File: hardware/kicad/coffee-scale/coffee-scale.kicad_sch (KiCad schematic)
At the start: 0 parts

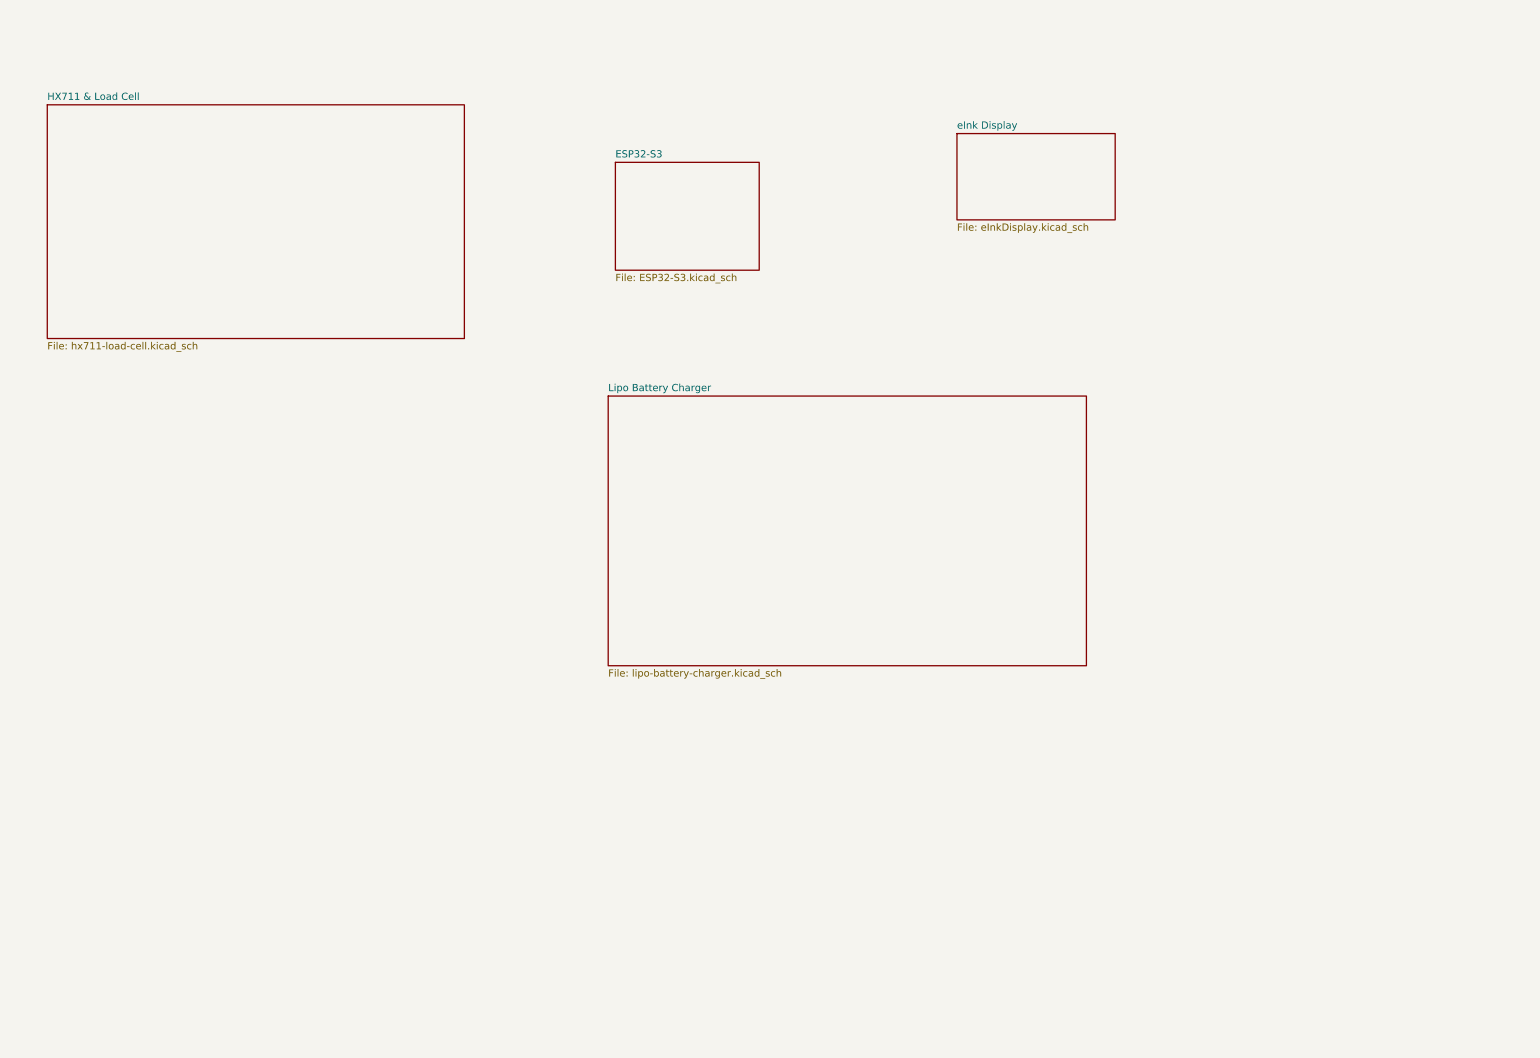
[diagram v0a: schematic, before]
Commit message: Create 10-31-24.md
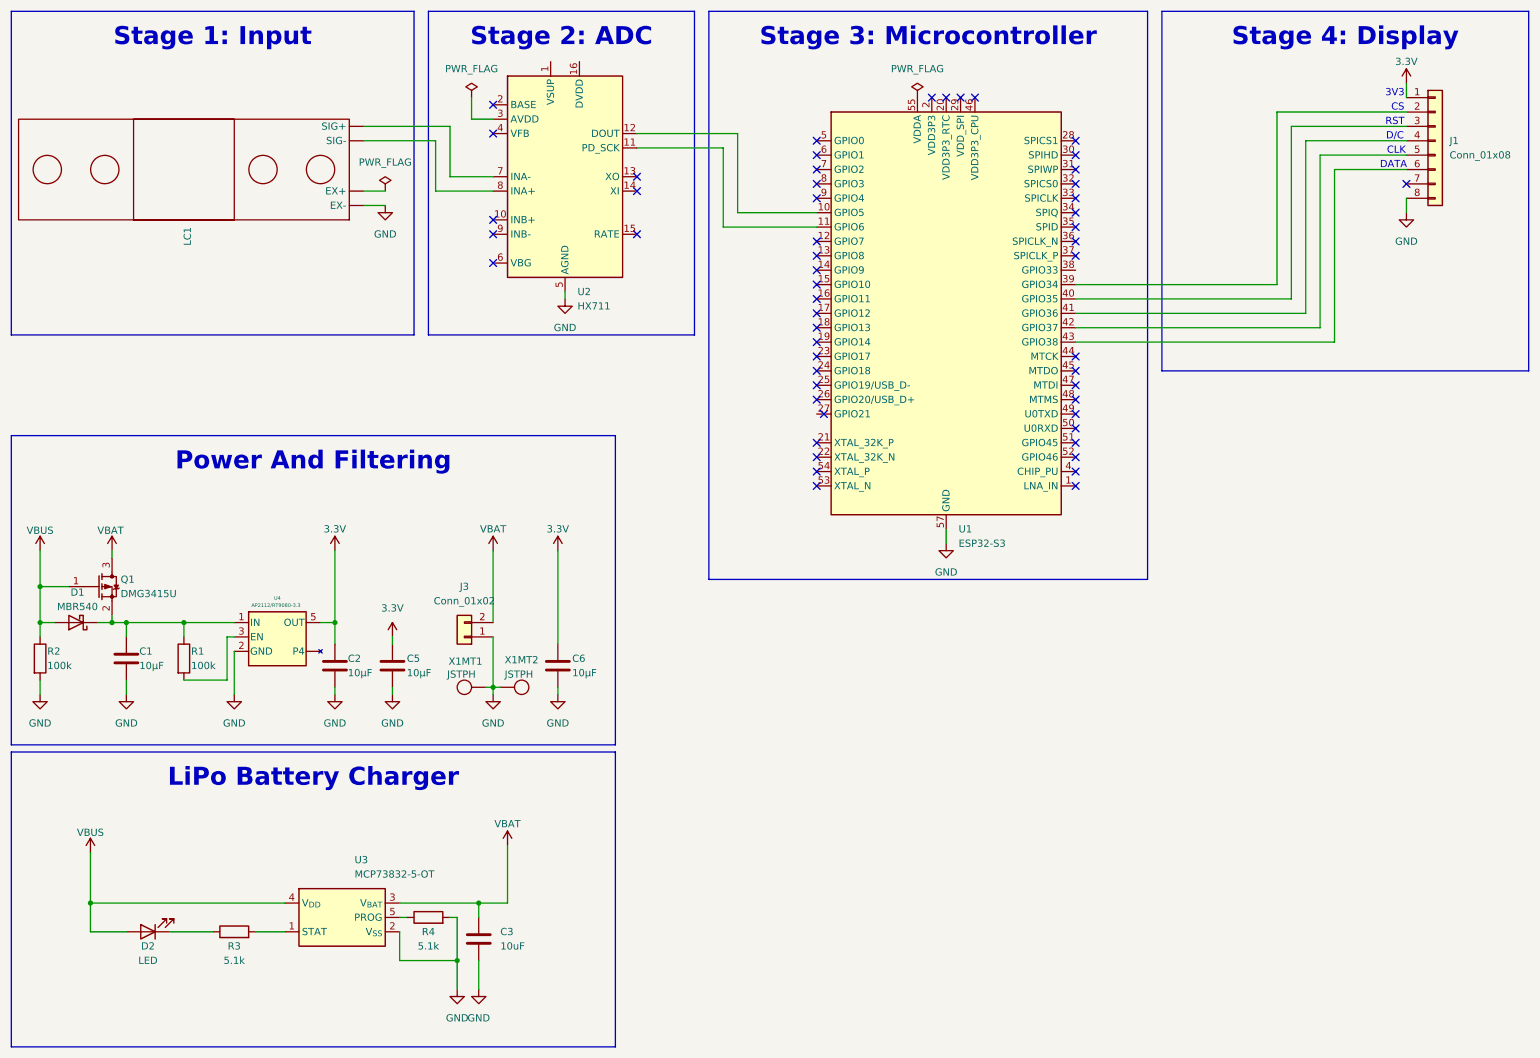
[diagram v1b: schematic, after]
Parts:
- added C1, C2, C5, C6: 10μF, symbol Device:C
- added C3: 10uF, symbol Device:C
- added D1: MBR540, Diode_THT:D_DO-201AD_P15.24mm_Horizontal, symbol Diode:MBR340
- added D2: LED, symbol Device:LED
- added J1: Conn_01x08, symbol Connector_Generic:Conn_01x08
- added J3: Conn_01x02, symbol Connector_Generic:Conn_01x02
- added LC1: ~, symbol Custom:4540
- added Q1: DMG3415U, Package_TO_SOT_SMD:SOT-23, symbol Transistor_FET:DMG2301L
- added R1, R2: 100k, symbol Device:R
- added R3, R4: 5.1k, symbol Device:R
- added U1: ESP32-S3, Package_DFN_QFN:QFN-56-1EP_7x7mm_P0.4mm_EP4x4mm, symbol MCU_Espressif:ESP32-S3
- added U2: HX711, Package_SO:SOP-16_3.9x9.9mm_P1.27mm, symbol Analog_ADC:HX711
- added U3: MCP73832-5-OT, Package_TO_SOT_SMD:SOT-23-5, symbol Battery_Management:MCP73832-5-OT
- added U4: AP2112/RT9080-3.3, Package_TO_SOT_SMD:SOT-23-5, symbol Regulator_Linear:AP2112K-1.2
- added X1MT1: JSTPH, symbol Connector:Conn_01x02_Socket
- added X1MT2: JSTPH, symbol Connector:Conn_01x01_Socket
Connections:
- new net: LC1. (SIG-), U2.7 (INA-)
- new net: LC1. (SIG-), U2.8 (INA+)
- new net: R3.2, U3.1 (STAT)
- new net: R4.1, U3.5 (PROG)
- new net: C1.1, D1.1 (K), Q1.2 (S), R1.1, U4.1 (IN)
- new net: R1.2, U4.3 (EN)
- new net: U1.10 (GPIO5), U2.12 (DOUT)
- new net: U1.11 (GPIO6), U2.11 (PD_SCK)
- new net: U1.2 (VDD3P3), U1.3 (VDD3P3)
- new net: J1.2 (Pin_2), U1.39 (GPIO34)
- new net: J1.3 (Pin_3), U1.40 (GPIO35)
- new net: J1.4 (Pin_4), U1.41 (GPIO36)
- new net: J1.5 (Pin_5), U1.42 (GPIO37)
- new net: J1.6 (Pin_6), U1.43 (GPIO38)
- new net: U1.55 (VDDA), U1.56 (VDDA)
- new net: D2.1 (K), R3.1
- new net 3.3V: C2.1, C5.1, C6.1, J1.1 (Pin_1), U4.5 (OUT)
- new net GND: C1.2, C2.2, C3.2, C5.2, C6.2, J1.8 (Pin_8), J3.1 (Pin_1), LC1. (SIG-), R2.2, R4.2, U1.57 (GND), U2.5 (AGND), U3.2 (V_{SS}), U4.2 (GND), X1MT1., X1MT2.
- new net VBAT: C3.1, J3.2 (Pin_2), Q1.3 (D), U3.3 (V_{BAT})
- new net VBUS: D1.2 (A), D2.2 (A), Q1.1 (G), R2.1, U3.4 (V_{DD})
- no-connect marks 0 -> 54
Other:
- removed sheet ESP32-S3
- removed sheet HX711 & Load Cell
- removed sheet Lipo Battery Charger
- removed sheet eInk Display
- note added: "3V3"
- note added: "CLK"
- note added: "CS"
- note added: "D/C"
- note added: "DATA"
- note added: "RST"
